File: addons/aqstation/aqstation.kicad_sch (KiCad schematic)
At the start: 8 parts, among them J1 PMSA003, J2 Conn_02x06_Odd_Even, J3 Adafruit_I2C_Header, J5 RGB_Header, J6 Pimoroni_I2CGarden_Header, J7 StemmaQT_Qwiic_Header, J8 BME680_Header

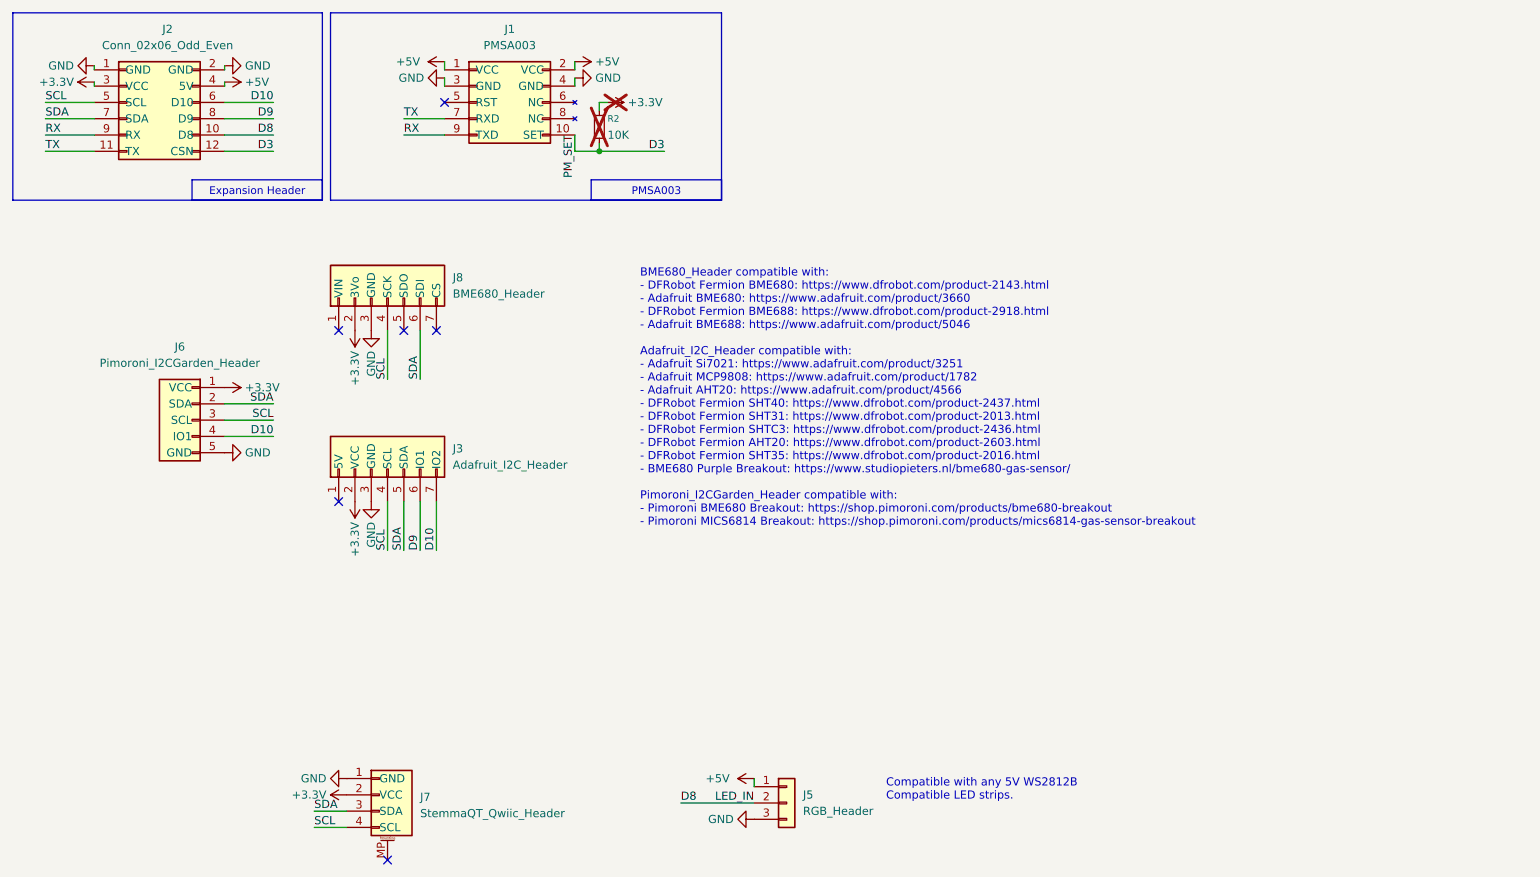
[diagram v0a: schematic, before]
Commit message: Finalize aqstation
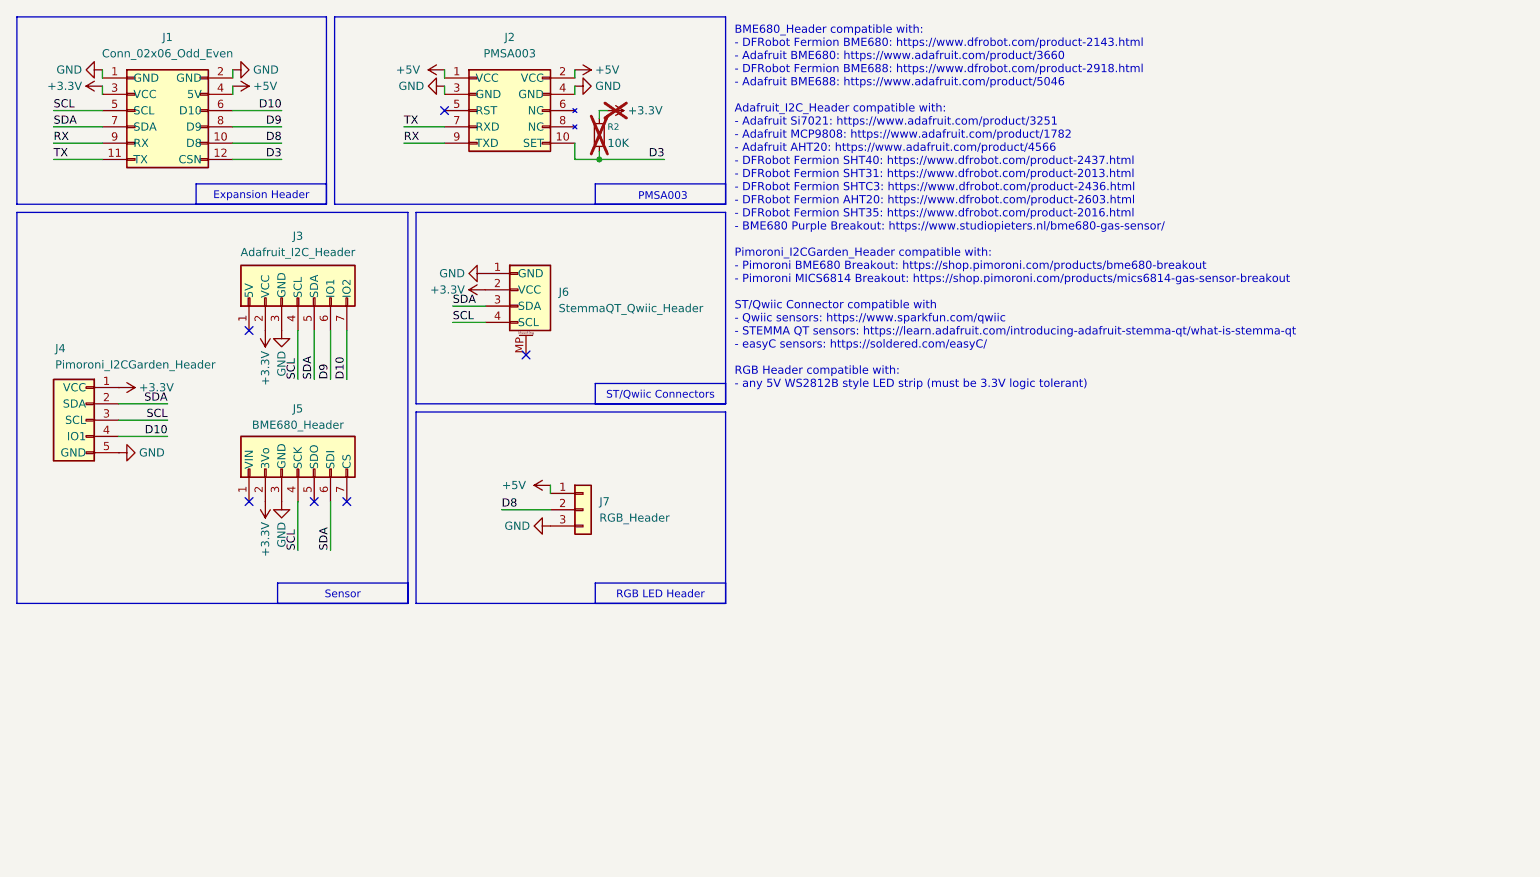
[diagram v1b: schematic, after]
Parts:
- renumbered J2 to J1, J1 to J2, J6 to J4, J8 to J5, J7 to J6, J5 to J7
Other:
- note added: "RGB LED Header"
- note added: "ST/Qwiic Connectors"
- note added: "Sensor"
- note removed: "Compatible with any 5V WS2812B Compatible LED strips."
- moved on the sheet: J1, J2, J3, J4, J5, J6, J7, R2
